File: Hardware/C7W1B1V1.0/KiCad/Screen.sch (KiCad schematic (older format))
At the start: 3 parts, among them J1 Waveshare 12955

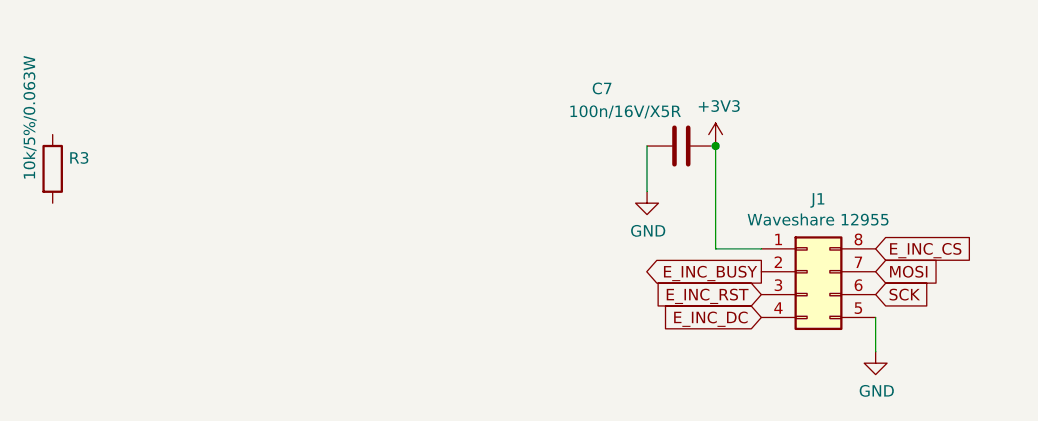
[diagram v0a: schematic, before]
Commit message: Dodano projekt Cube
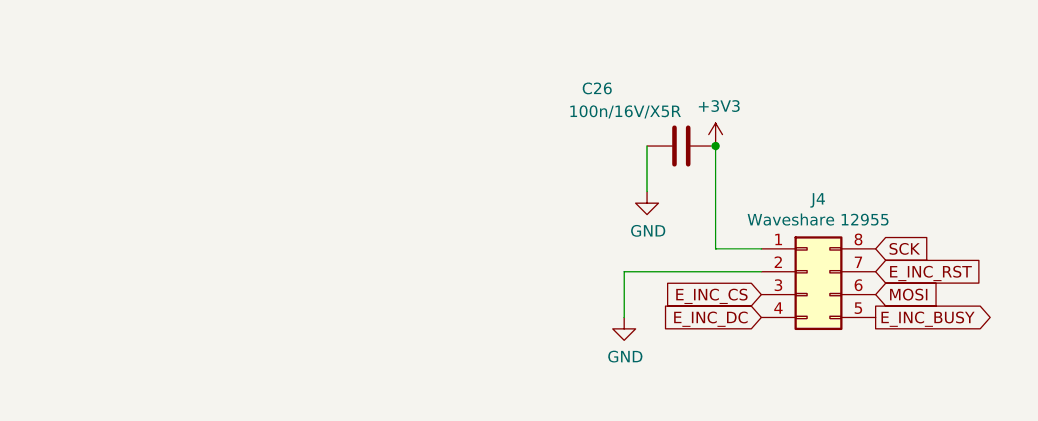
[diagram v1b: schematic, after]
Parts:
- removed R3: 10k/5%/0.063W, Resistor_SMD:R_0402_1005Metric, symbol Device:R
- renumbered C7 to C26, J1 to J4
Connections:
- net E_INC_BUSY: now also J4.5 (Pin_5); no longer J4.2 (Pin_2)
- net E_INC_CS: now also J4.3 (Pin_3); no longer J4.8 (Pin_8)
- net E_INC_RST: now also J4.7 (Pin_7); no longer J4.3 (Pin_3)
- net GND: now also J4.2 (Pin_2); no longer J4.5 (Pin_5)
- net MOSI: now also J4.6 (Pin_6); no longer J4.7 (Pin_7)
- net SCK: now also J4.8 (Pin_8); no longer J4.6 (Pin_6)
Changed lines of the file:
@@
 $EndDescr
 $Comp
-L Connector_Generic:Conn_02x04_Counter_Clockwise J1
+L Connector_Generic:Conn_02x04_Counter_Clockwise J4
 U 1 1 672EF0FD
 P 4500 3300
-F 0 "J1" H 4550 3617 50  0000 C CNN
+F 0 "J4" H 4550 3617 50  0000 C CNN
 F 1 "Waveshare 12955" H 4550 3526 50  0000 C CNN
 F 2 "Connector_PinHeader_2.54mm:PinHeader_2x04_P2.54mm_Vertical" H 4500 3300 50  0001 C CNN
@@
 P 3950 2750
 AR Path="/672E4D00/672F0E30" Ref="C?"  Part="1"
-AR Path="/672EED17/672F0E30" Ref="C7"  Part="1"
-F 0 "C7" V 4200 3050 50  0000 L CNN
+AR Path="/672EED17/672F0E30" Ref="C26"  Part="1"
+F 0 "C26" V 4200 3050 50  0000 L CNN
 F 1 "100n/16V/X5R" V 4100 2750 50  0000 L CNN
 F 2 "Capacitor_SMD:C_0402_1005Metric" H 3988 2600 50  0001 C CNN
@@
 	0    -1   -1   0
 $EndComp
-$Comp
-L Device:R R?
-U 1 1 672F0E36
-P 1200 2850
-AR Path="/672E4D00/672F0E36" Ref="R?"  Part="1"
-AR Path="/672EED17/672F0E36" Ref="R3"  Part="1"
-F 0 "R3" H 1270 2896 50  0000 L CNN
-F 1 "10k/5%/0.063W" V 1100 2800 50  0000 L CNN
-F 2 "Resistor_SMD:R_0402_1005Metric" V 1130 2850 50  0001 C CNN
-F 3 "~" H 1200 2850 50  0001 C CNN
-	1    1200 2850
-	1    0    0    -1
-$EndComp
 Wire Wire Line
 	3800 2750 3800 2950
 $Comp
-L power:+3V3 #PWR0107
+L power:+3V3 #PWR060
 U 1 1 672F2716
 P 4100 2750
-F 0 "#PWR0107" H 4100 2600 50  0001 C CNN
+F 0 "#PWR060" H 4100 2600 50  0001 C CNN
 F 1 "+3V3" H 4115 2923 50  0000 C CNN
 F 2 "" H 4100 2750 50  0001 C CNN
@@
 Connection ~ 4100 2750
 $Comp
-L power:GND #PWR0108
+L power:GND #PWR059
 U 1 1 672F313E
 P 3800 2950
-F 0 "#PWR0108" H 3800 2700 50  0001 C CNN
+F 0 "#PWR059" H 3800 2700 50  0001 C CNN
 F 1 "GND" H 3805 2777 50  0000 C CNN
 F 2 "" H 3800 2950 50  0001 C CNN
@@
 $EndComp
 $Comp
-L power:GND #PWR0109
+L power:GND #PWR061
 U 1 1 672F3B6D
-P 4800 3650
-F 0 "#PWR0109" H 4800 3400 50  0001 C CNN
-F 1 "GND" H 4805 3477 50  0000 C CNN
-F 2 "" H 4800 3650 50  0001 C CNN
-F 3 "" H 4800 3650 50  0001 C CNN
-	1    4800 3650
+P 3700 3500
+F 0 "#PWR061" H 3700 3250 50  0001 C CNN
+F 1 "GND" H 3705 3327 50  0000 C CNN
+F 2 "" H 3700 3500 50  0001 C CNN
+F 3 "" H 3700 3500 50  0001 C CNN
+	1    3700 3500
 	1    0    0    -1
 $EndComp
-Wire Wire Line
-	4800 3500 4800 3650
-Text GLabel 4300 3300 0    50   Output ~ 0
+Text GLabel 4800 3500 2    50   Output ~ 0
 E_INC_BUSY
-Text GLabel 4300 3400 0    50   Input ~ 0
+Text GLabel 4800 3300 2    50   Input ~ 0
 E_INC_RST
 Text GLabel 4300 3500 0    50   Input ~ 0
 E_INC_DC
+Text GLabel 4300 3400 0    50   Input ~ 0
+E_INC_CS
+Text GLabel 4800 3400 2    50   Input ~ 0
+MOSI
 Text GLabel 4800 3200 2    50   Input ~ 0
-E_INC_CS
-Text GLabel 4800 3300 2    50   Input ~ 0
-MOSI
-Text GLabel 4800 3400 2    50   Input ~ 0
 SCK
+Wire Wire Line
+	4300 3300 3700 3300
+Wire Wire Line
+	3700 3300 3700 3500
 $EndSCHEMATC
